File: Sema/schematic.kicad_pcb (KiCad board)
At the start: 2 copper layers, 114 x 82.8 mm, 73 parts, among them J1 Conn_01x05_Male, J10 Conn_01x05_Male, J11 Conn_01x03_Male, J12 Conn_01x03_Male, J2 Conn_01x05_Male, J4 USB_B, J5 Conn_01x05_Male, J6 Conn_01x05_Male, J7 Conn_01x05_Male, J8 Conn_01x05_Male, J9 Conn_01x05_Male, U1 PIC24FJ64GA702-I/SO, U10 74LVT573MTC, U11 ULN2003AIDR, U12 ULN2003AIDR, U13 ULN2003AIDR, U14 ULN2003AIDR, U2 ABLS-8.000MHZ-B2-T, U3 FT232RL, U3.3V1 LM317BTG, U4 CD74HC4514M96, U5 74LVT573MTC, U6 74LVT573MTC, U7 74LVT573MTC, U8 74LVT573MTC, U9 74LVT573MTC

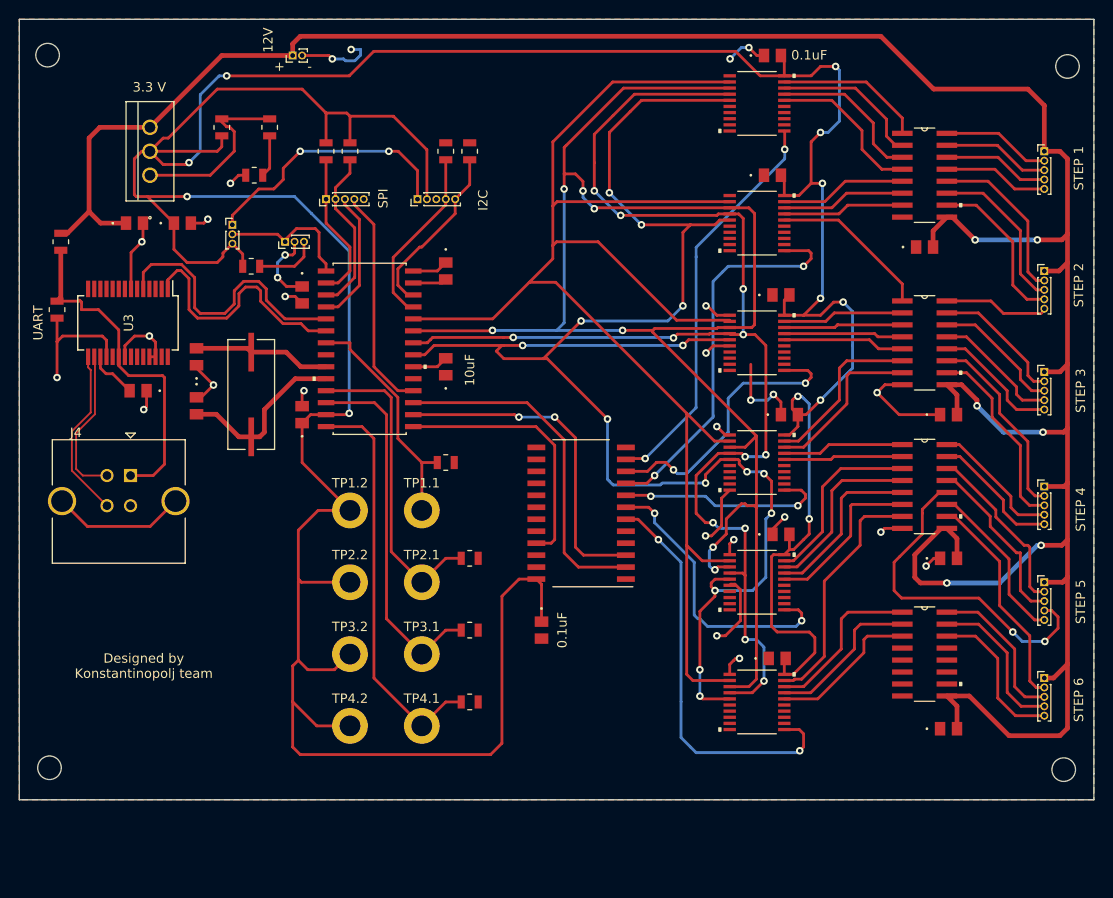
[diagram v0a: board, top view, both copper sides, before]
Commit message: Finalna verzija layout-a
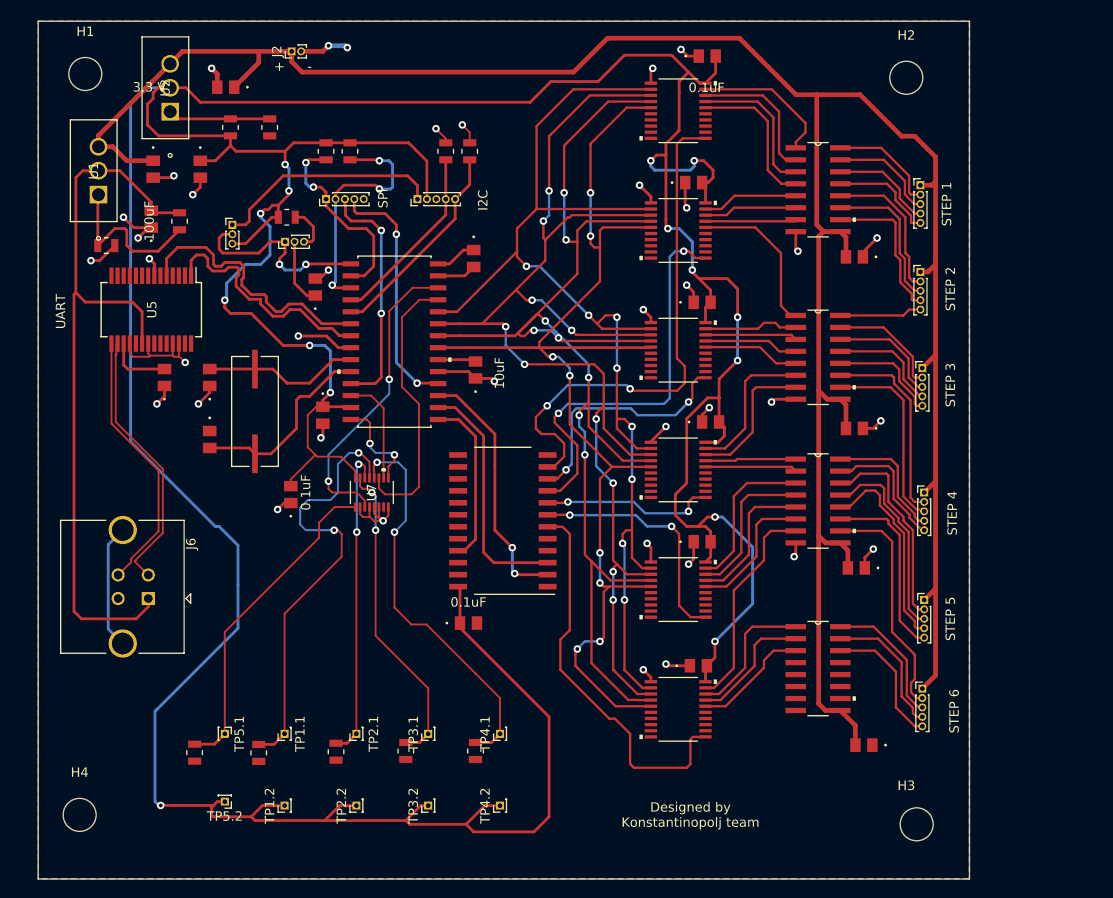
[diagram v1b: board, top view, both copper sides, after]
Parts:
- removed 12V: Conn_01x02_Male, Connector_PinHeader_1.00mm:PinHeader_1x02_P1.00mm_Vertical
- removed the R9 at (50.6, 60.4)
- removed U3.3V1: LM317BTG, LM317BTGj:LM317BTG
- added C1: 0.1uF, footprints:08055A220JAT2A, F.Cu at (60.4, 52.7)
- added C13: 0.1uF, footprints:08055A220JAT2A, F.Cu at (75.0, 87.2)
- added C2: 100uF, footprints:08055A220JAT2A, F.Cu at (60.2, 58.0)
- added J2: Conn_01x02_Male, Connector_PinHeader_1.00mm:PinHeader_1x02_P1.00mm_Vertical, F.Cu at (75.1, 40.2)
- added R14: 10k, HCJ0805ZT0R00j:HCJ0805ZT0R00, F.Cu at (64.8, 114.6)
- added TP5.1: TestPoint_Small, Connector_PinHeader_1.00mm:PinHeader_1x01_P1.00mm_Vertical, F.Cu at (68.0, 112.6)
- added TP5.2: TestPoint_Small, Connector_PinHeader_1.00mm:PinHeader_1x01_P1.00mm_Vertical, F.Cu at (68.0, 119.8)
- added U1: LM317AT/NOPB, LM317AT:LM317AT, F.Cu at (54.6, 55.4)
- added U2: LM317AT/NOPB, LM317AT:LM317AT, F.Cu at (62.2, 46.6)
- added U7: PTMUX1308QDYYRQ1, PTMUX1308QDYYRQ1j:PTMUX1308QDYYRQ1, F.Cu at (83.6, 87.0)
- C7: renamed from C5; value 22uf -> 100uf
- C8: renamed from C6; value 22uF -> 0.1uF
- H1, H2, H3, H4: footprint MountingHole:MountingHole_2.5mm -> MountingHole:MountingHole_3.5mm
- R3: value 12k -> 270
- R4: renamed from R8; value 10k -> 820
- TP1.1, TP1.2, TP2.1, TP2.2, TP3.1, TP3.2, TP4.1, TP4.2: footprint MountingHole:MountingHole_2.2mm_M2_DIN965_Pad -> Connector_PinHeader_1.00mm:PinHeader_1x01_P1.00mm_Vertical
- moved R10 36.6 mm to (71.6, 114.6), turned to 90 degrees
- moved TP1.2 32.1 mm to (74.3, 120.2), turned to 90 degrees
- moved TP1.1 27.8 mm to (74.3, 112.6), turned to 90 degrees
- moved R11 24.9 mm to (79.8, 114.5), turned to 90 degrees
- moved TP2.2 23.7 mm to (82.0, 120.2), turned to 90 degrees
- moved TP3.2 18.1 mm to (89.6, 120.2), turned to 90 degrees
- moved TP4.2 18.0 mm to (97.2, 120.2), turned to 90 degrees
- moved TP2.1 17.5 mm to (82.0, 112.6), turned to 90 degrees
- moved C8 17.4 mm to (68.1, 44.0), turned to 180 degrees
- moved H2 17.1 mm to (140.3, 43.0)
- moved H3 16.6 mm to (141.4, 122.2)
- moved R12 14.5 mm to (87.2, 114.4), turned to 90 degrees
- moved J7 13.6 mm to (141.8, 54.4)
- moved J6 13.2 mm to (59.9, 98.2), turned to -90 degrees
- moved J8 13.1 mm to (141.8, 63.6)
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- renumbered C8 to C10, C9 to C11, C10 to C12, C11 to C14, C12 to C15, C13 to C16, C14 to C17, C15 to C18, C16 to C19, C17 to C20, C18 to C21, C19 to C22, C1 to C3, C2 to C4, C3 to C5, C4 to C6, C7 to C9, J8 to J10, J9 to J11, J10 to J12, J11 to J3, J2 to J4, J12 to J5, J4 to J6, J5 to J7, J6 to J8, J7 to J9, R4 to R5, R5 to R6, R14 to R7, R6 to R8, R7 to R9, U7 to U10, U8 to U11, U9 to U12, U10 to U13, U11 to U14, U12 to U15, U13 to U16, U14 to U17, U1 to U3, U2 to U4, U3 to U5, U4 to U6, U5 to U8, U6 to U9
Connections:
- R3 pad 2: GND -> 5V
- R4 pad 2: 5V -> Net-(R3-Pad1)
- R5 pad 1: Net-(R3-Pad1) -> GND
- U3 pad 11: P2 -> MISO
- U3 pad 12: P3 -> S1
- U3 pad 14: P4 -> S2
- U3 pad 25: PGD -> S0
- U3 pad 26: PGC -> M
- U3 pad 4: MISO -> PGD
- U3 pad 5: tx -> PGC
- U3 pad 6: RX -> tx
- U3 pad 7: P1 -> RX
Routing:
- net D4: track 172.6 -> 122.6 mm, vias 14 -> 8
- net 5V: track 36.4 -> 80.6 mm
- net 3.3V: track 428.2 -> 471.7 mm, vias 12 -> 15
- net D2: track 171.5 -> 135.6 mm, vias 7 -> 10
- net P5: track 0.00 -> 34.7 mm
- net D1: track 158.7 -> 125.4 mm, vias 0 -> 8
- net M: track 0.00 -> 32.8 mm, vias 0 -> 2
- net S0: track 0.00 -> 29.3 mm
- net 12V: track 292.4 -> 267.7 mm, vias 6 -> 0
- net P1: track 25.1 -> 47.1 mm, vias 0 -> 2
- net PI5: track 36.6 -> 21.6 mm, vias 2 -> 0
- net Net-(R3-Pad1): track 4.49 -> 17.7 mm
- net E1: track 43.0 -> 55.3 mm
- net D-: track 16.3 -> 28.5 mm
- net S1: track 0.00 -> 11.4 mm
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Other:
- board size 114 x 82.8 mm -> 98.8 x 91 mm
